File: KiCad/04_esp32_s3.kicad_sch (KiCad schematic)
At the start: 1 part, among them IC101 ESP32-S3-WROOM-1-N16R8

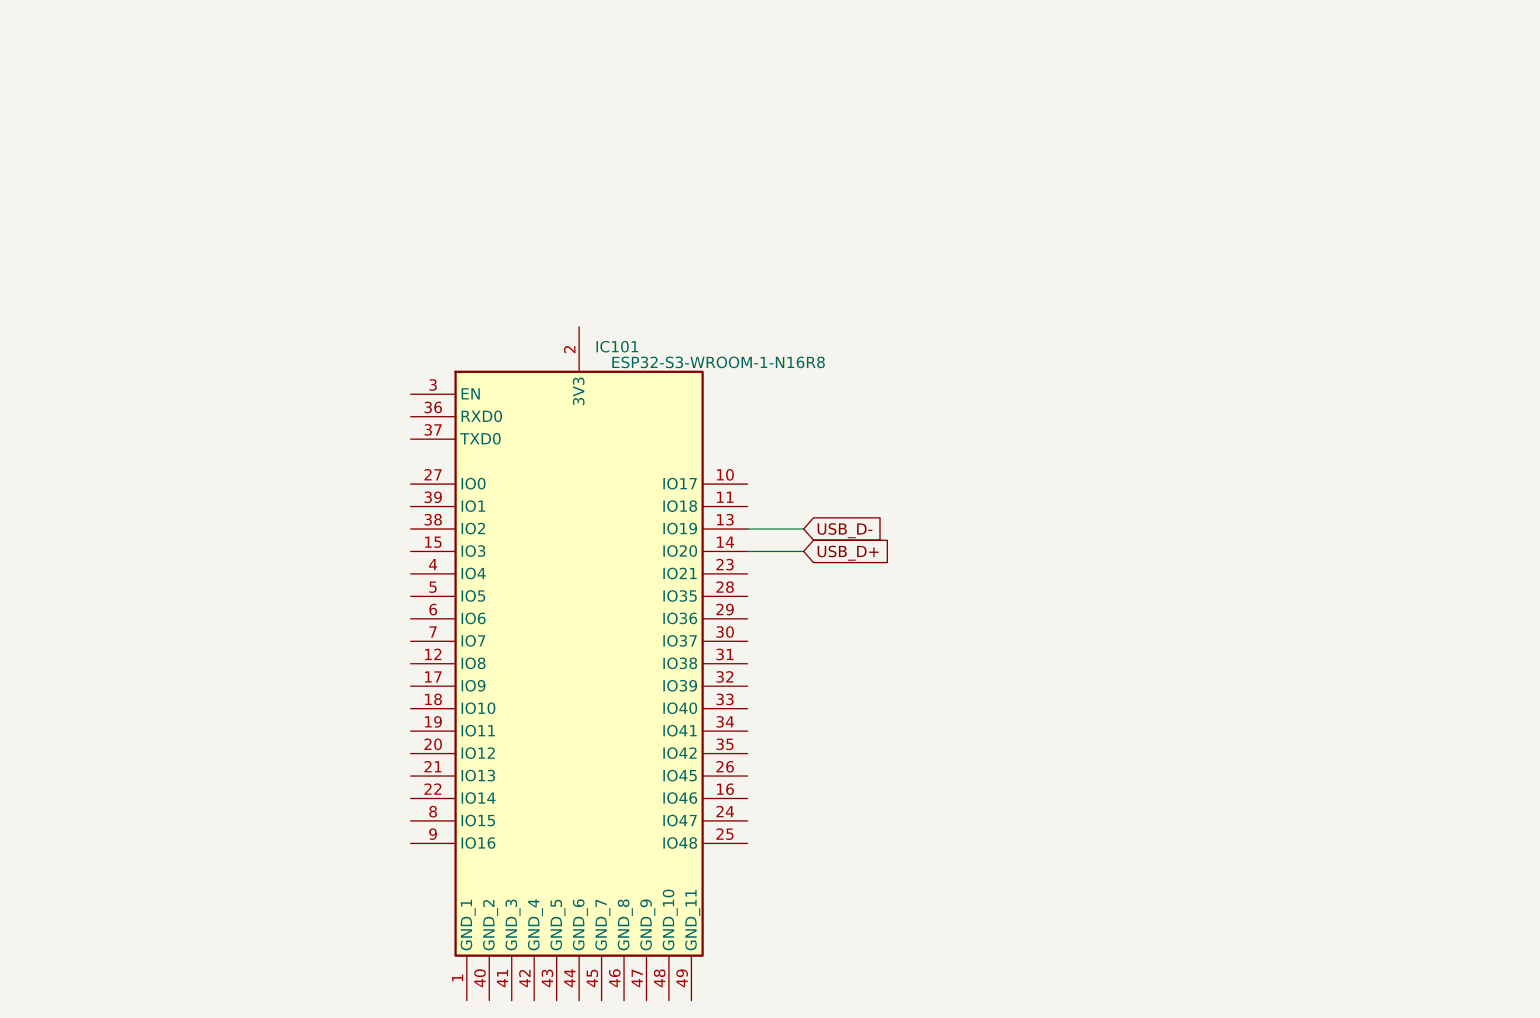
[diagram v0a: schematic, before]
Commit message: Update power scheme
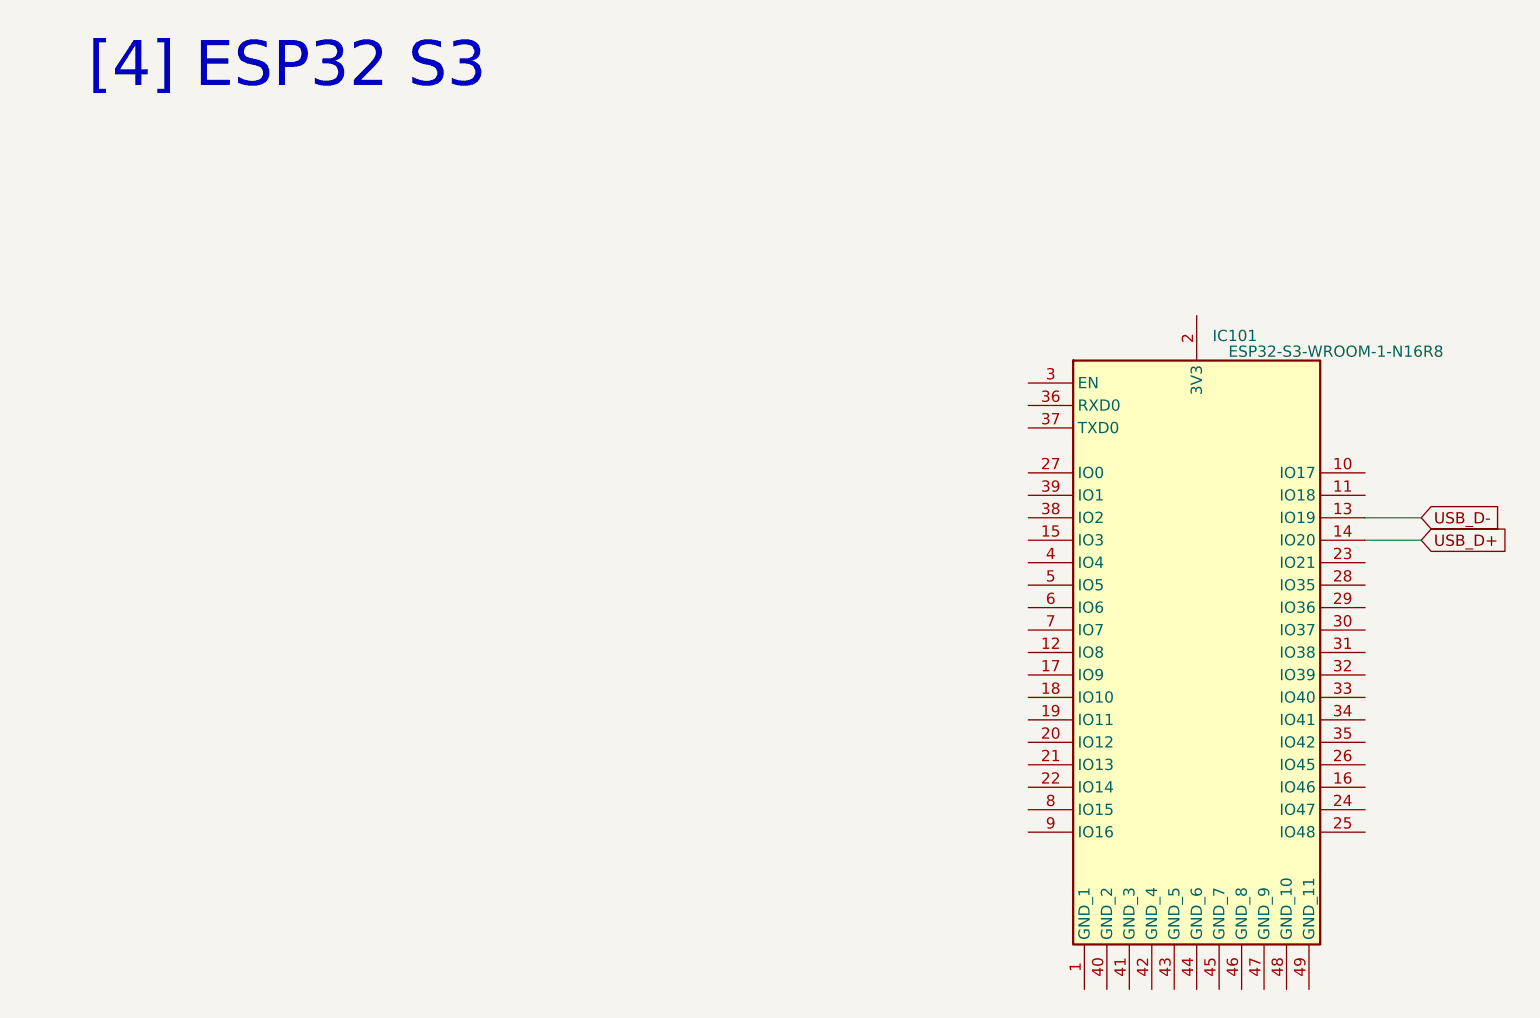
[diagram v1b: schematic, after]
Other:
- note added: "[4] ESP32 S3"
- moved on the sheet: IC101
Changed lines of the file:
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@@
 	(generator_version "9.0")
 	(paper "A4")
+	(text "[4] ESP32 S3"
+		(exclude_from_sim no)
+		(at 43.18 21.336 0)
+		(effects
+			(font
+				(size 5.08 5.08)
+			)
+		)
+	)
 	(wire
 		(pts
-			(xy 95.25 73.66) (xy 101.6 73.66)
+			(xy 165.1 72.39) (xy 171.45 72.39)
 		)
 		(stroke
@@
 	(wire
 		(pts
-			(xy 95.25 76.2) (xy 101.6 76.2)
+			(xy 165.1 74.93) (xy 171.45 74.93)
 		)
 		(stroke
@@
 	(global_label "USB_D+"
 		(shape input)
-		(at 101.6 76.2 0)
+		(at 171.45 74.93 0)
 		(fields_autoplaced yes)
 		(effects
@@
 		)
 		(property "Intersheetrefs" "${INTERSHEET_REFS}"
-			(at 112.2052 76.2 0)
+			(at 182.0552 74.93 0)
 			(effects
 				(font
@@
 	(global_label "USB_D-"
 		(shape input)
-		(at 101.6 73.66 0)
+		(at 171.45 72.39 0)
 		(fields_autoplaced yes)
 		(effects
@@
 		)
 		(property "Intersheetrefs" "${INTERSHEET_REFS}"
-			(at 112.2052 73.66 0)
+			(at 182.0552 72.39 0)
 			(effects
 				(font
@@
 	(symbol
 		(lib_id "esp32_s3_weather_webserver:ESP32-S3-WROOM-1-N16R8")
-		(at 62.23 55.88 0)
+		(at 132.08 54.61 0)
 		(unit 1)
 		(exclude_from_sim no)
@@
 		(dnp no)
 		(property "Reference" "IC101"
-			(at 80.518 53.086 0)
+			(at 150.368 51.816 0)
 			(effects
 				(font
@@
 		)
 		(property "Value" "ESP32-S3-WROOM-1-N16R8"
-			(at 91.948 54.864 0)
+			(at 161.798 53.594 0)
 			(effects
 				(font
@@
 		)
 		(property "Footprint" "esp32_s3_weather_webserver:ESP32S3WROOM1N16R8"
-			(at 91.44 150.8 0)
+			(at 161.29 149.53 0)
 			(effects
 				(font
@@
 		)
 		(property "Datasheet" "https://www.espressif.com/sites/default/files/documentation/esp32-s3-wroom-1_wroom-1u_datasheet_en.pdf"
-			(at 91.44 250.8 0)
+			(at 161.29 249.53 0)
 			(effects
 				(font
@@
 		)
 		(property "Description" "Multiprotocol Modules SMD Module, ESP32-S3R8, 3.3V, 8 MB Octal PSRAM Die, 16 MB Quad SPI Flash, PCB Antenna"
-			(at 73.406 167.64 0)
+			(at 143.256 166.37 0)
 			(effects
 				(font
@@
 		)
 		(property "Height" "3.25"
-			(at 91.44 450.8 0)
+			(at 161.29 449.53 0)
 			(effects
 				(font
@@
 		)
 		(property "Manufacturer_Name" "Espressif Systems"
-			(at 91.44 550.8 0)
+			(at 161.29 549.53 0)
 			(effects
 				(font
@@
 		)
 		(property "Manufacturer_Part_Number" "ESP32-S3-WROOM-1-N16R8"
-			(at 91.44 650.8 0)
+			(at 161.29 649.53 0)
 			(effects
 				(font
@@
 		)
 		(property "Mouser Part Number" "356-ESP32S3WRM1N16R8"
-			(at 91.44 750.8 0)
+			(at 161.29 749.53 0)
 			(effects
 				(font
@@
 		)
 		(property "Mouser Price/Stock" "https://www.mouser.co.uk/ProductDetail/Espressif-Systems/ESP32-S3-WROOM-1-N16R8?qs=Li%252BoUPsLEnvQc9gW6AMhZg%3D%3D"
-			(at 91.44 850.8 0)
+			(at 161.29 849.53 0)
 			(effects
 				(font
@@
 		)
 		(property "Arrow Part Number" ""
-			(at 91.44 950.8 0)
+			(at 161.29 949.53 0)
 			(effects
 				(font
@@
 		)
 		(property "Arrow Price/Stock" ""
-			(at 91.44 1050.8 0)
+			(at 161.29 1049.53 0)
 			(effects
 				(font
